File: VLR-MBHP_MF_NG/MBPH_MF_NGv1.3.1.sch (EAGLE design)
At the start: 51 parts, among them J40 MF_I/O, J41 MF_I/O to more MF_NG

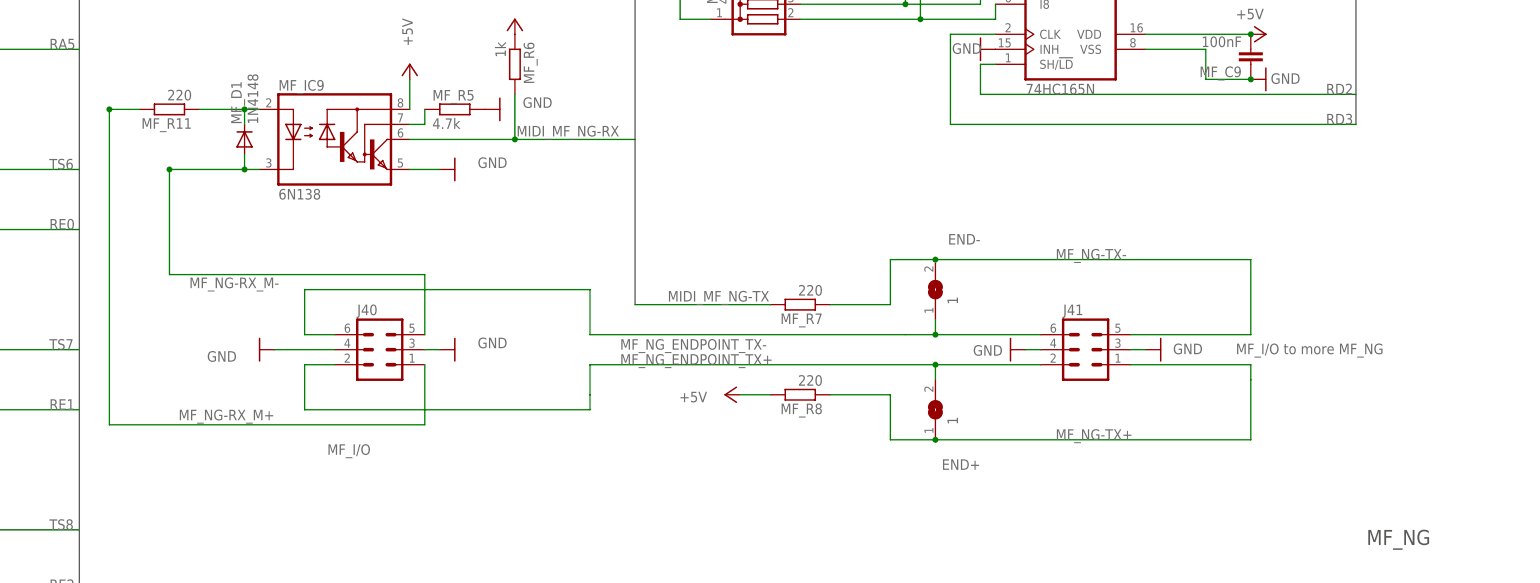
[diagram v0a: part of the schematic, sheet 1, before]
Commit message: div. changes
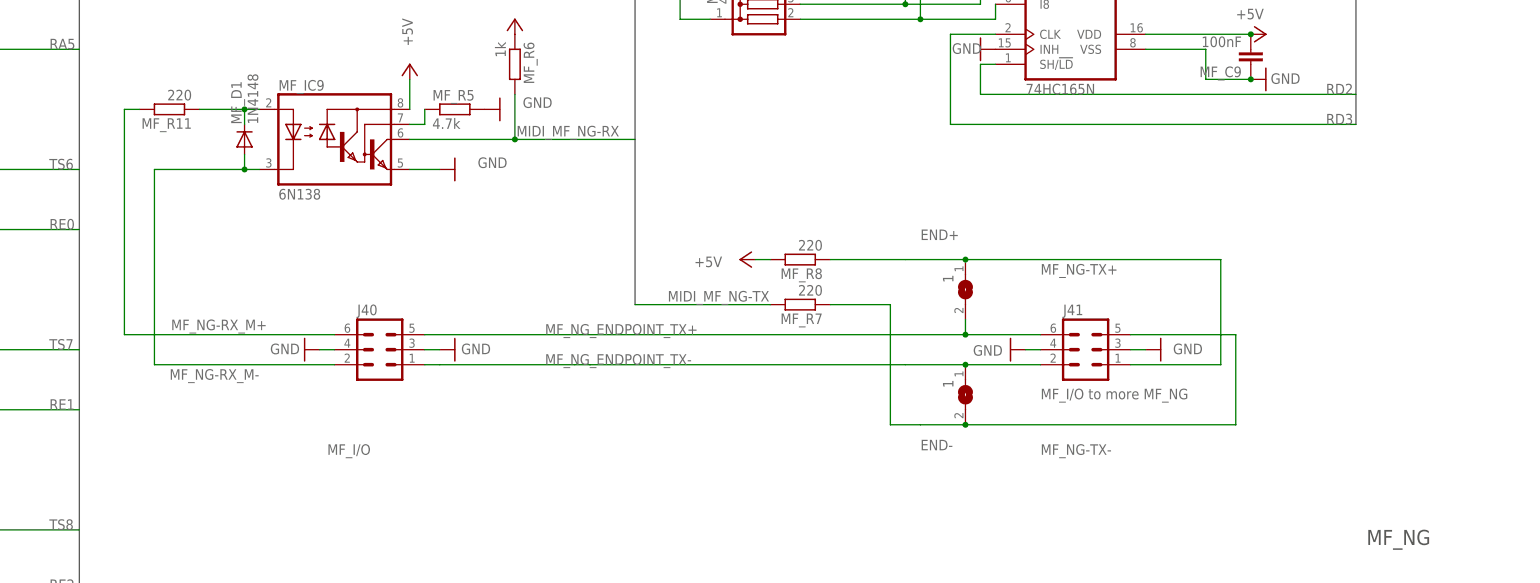
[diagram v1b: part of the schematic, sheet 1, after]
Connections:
- net MF_NG-RX_M+: now also J40.6; no longer J40.1
- net MF_NG-RX_M-: now also J40.2; no longer J40.5
- net MF_NG_ENDPOINT_TX+: now also J40.5, J41.6; no longer J40.2, J41.2
- net MF_NG_ENDPOINT_TX-: now also J40.1, J41.2; no longer J40.6, J41.6
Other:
- moved on the sheet: END+, END-, MF_R8
